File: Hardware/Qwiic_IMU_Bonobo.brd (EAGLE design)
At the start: 30.5 x 25.4 mm, 89 parts, among them J2 SMD, J3 PTH, J4 SMD, J6 SPI, U2 BNO080, Y1 32.768kHz

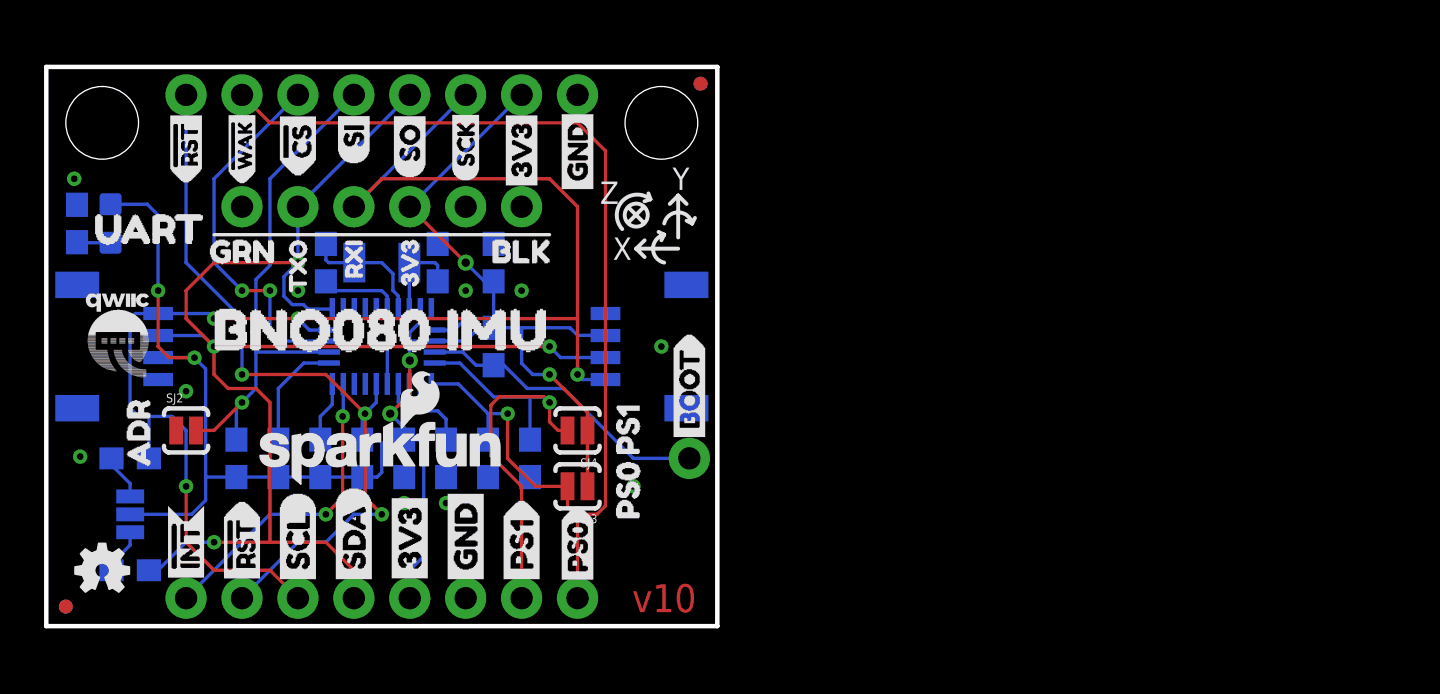
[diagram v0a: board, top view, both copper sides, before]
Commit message: Adding panel files
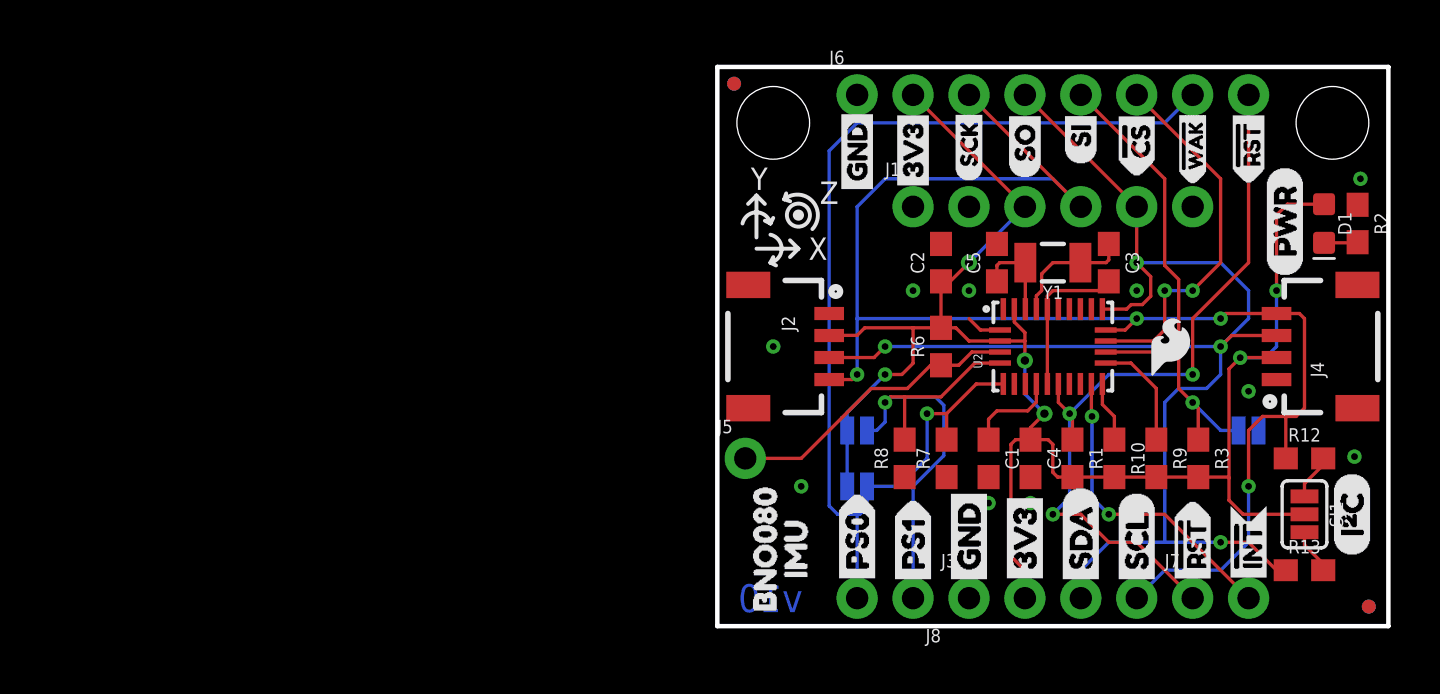
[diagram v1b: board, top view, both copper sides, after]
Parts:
- moved JP1 59.2 mm to (29.6, 0.89), flipped to the bottom
- moved JP2 59.2 mm to (29.6, 0.89), flipped to the top
- moved U$39 58.9 mm to (29.5, 18.0), flipped to the bottom
- moved R2 58.2 mm to (29.1, 18.3), flipped to the top
- moved U$23 57.7 mm to (28.8, 3.17), flipped to the top
- moved JP4 55.9 mm to (27.9, 22.9), flipped to the top
- moved LOGO1 55.9 mm to (27.9, 2.54), flipped to the bottom
- moved D1 55.1 mm to (27.6, 18.3), flipped to the top
- moved U$59 54.6 mm to (27.3, 13.2), flipped to the bottom
- moved R12 53.3 mm to (26.7, 7.62), flipped to the top
- moved R13 53.3 mm to (26.7, 2.54), flipped to the top
- moved SJ1 53.3 mm to (26.7, 5.08), flipped to the top
- moved U$30 52.6 mm to (26.3, 6.35), flipped to the bottom
- moved U$1 51.6 mm to (25.8, 15.9), flipped to the top
- moved J4 50.8 mm to (25.4, 12.7), flipped to the top
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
